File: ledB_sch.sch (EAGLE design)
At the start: 6 parts, among them IC1 LM741P

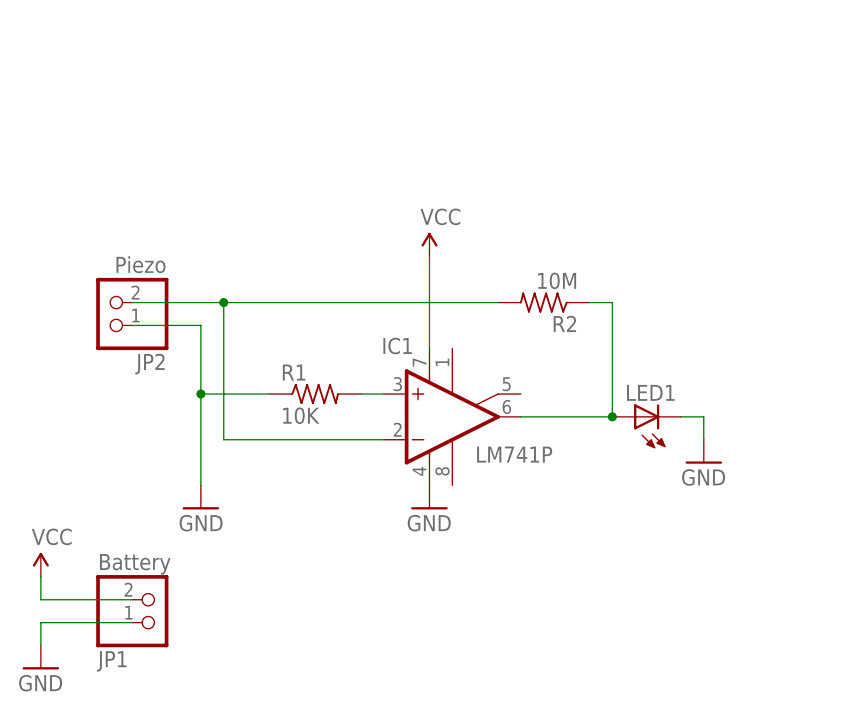
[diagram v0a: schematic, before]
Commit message: fix schema, one layer round design
and fixed the schema
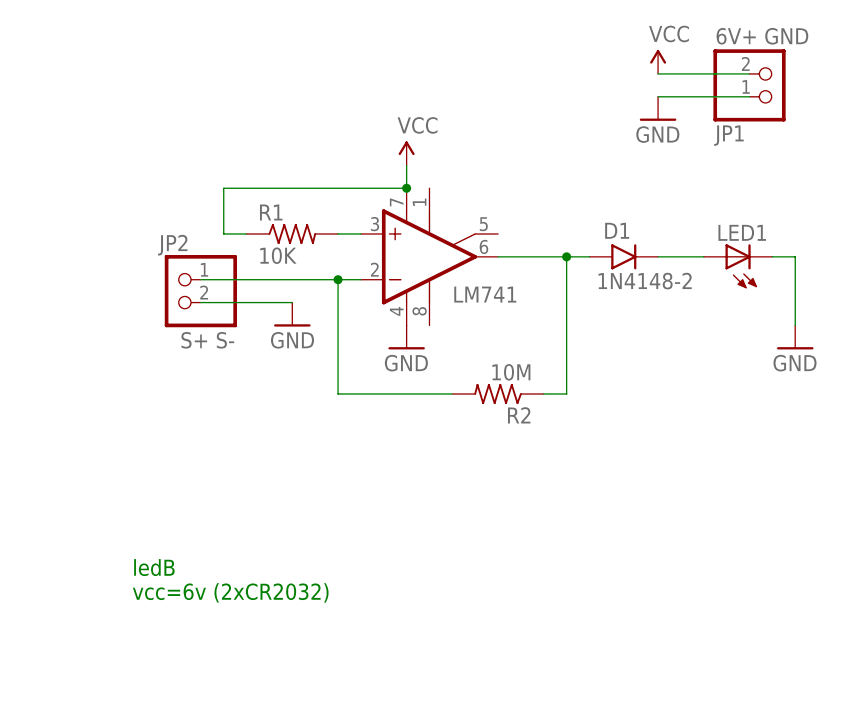
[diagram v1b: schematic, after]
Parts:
- removed IC1: LM741P, linear:LM741P
- added D1: 1N4148-2, gm-diodes:1N4148-2
- added OPAMP: LM741, linear:LM741P
- JP1: value Battery -> 6V+ GND
- JP2: value Piezo -> S+ S-
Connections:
- removed net N$3: IC1.-IN, JP2.2, R2.2
- new net N$5: D1.C, LED1.A
- new net SIG: JP2.1, OPAMP.-IN, R2.2
- net GND: now also JP2.2, OPAMP.V-; no longer IC1.V-, JP2.1, R1.1
- net N$1: now also OPAMP.+IN; no longer IC1.+IN
- net N$2: now also D1.A, OPAMP.OUT; no longer IC1.OUT, LED1.A
- net VCC: now also OPAMP.V+, R1.1; no longer IC1.V+
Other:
- note added: "ledB vcc=6v (2xCR2032)"
- moved on the sheet: JP1, JP2, LED1, R1, R2
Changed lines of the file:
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@@
 <?xml version="1.0" encoding="utf-8"?>
 <!DOCTYPE eagle SYSTEM "eagle.dtd">
-<eagle version="6.3">
+<eagle version="7.1.0">
 <drawing>
 <settings>
@@
 <setting verticaltext="up"/>
 </settings>
-<grid distance="0.1" unitdist="inch" unit="mil" style="lines" multiple="1" display="no" altdistance="0.01" altunitdist="inch" altunit="inch"/>
+<grid distance="0.1" unitdist="inch" unit="inch" style="lines" multiple="1" display="no" altdistance="0.01" altunitdist="inch" altunit="inch"/>
 <layers>
 <layer number="1" name="Top" color="4" fill="1" visible="no" active="no"/>
@@
 </classes>
 <parts>
-<part name="IC1" library="linear" deviceset="*741" device="P" technology="LM"/>
+<part name="OPAMP" library="linear" deviceset="*741" device="P" technology="LM" value="LM741"/>
 <part name="R1" library="adafruit" deviceset="R-US_" device="0207/7" value="10K"/>
 <part name="R2" library="adafruit" deviceset="R-US_" device="0207/7" value="10M"/>
 <part name="LED1" library="SparkFun-LED" deviceset="LED" device="5MM"/>
-<part name="P+1" library="SparkFun-Aesthetics" deviceset="VCC" device=""/>
-<part name="GND1" library="SparkFun-Aesthetics" deviceset="GND" device=""/>
-<part name="GND3" library="SparkFun-Aesthetics" deviceset="GND" device=""/>
 <part name="GND4" library="SparkFun-Aesthetics" deviceset="GND" device=""/>
-<part name="JP1" library="microbuilder" deviceset="HEADER-1X2" device="" value="Battery"/>
-<part name="JP2" library="microbuilder" deviceset="HEADER-1X2" device="" value="Piezo"/>
+<part name="JP1" library="microbuilder" deviceset="HEADER-1X2" device="" value="6V+     GND"/>
+<part name="JP2" library="microbuilder" deviceset="HEADER-1X2" device="" value="S+     S-"/>
 <part name="P+2" library="SparkFun-Aesthetics" deviceset="VCC" device=""/>
 <part name="GND2" library="SparkFun-Aesthetics" deviceset="GND" device=""/>
+<part name="D1" library="gm-diodes" deviceset="1N4148" device="-2"/>
+<part name="GND1" library="SparkFun-Aesthetics" deviceset="GND" device=""/>
+<part name="P+3" library="SparkFun-Aesthetics" deviceset="VCC" device=""/>
+<part name="GND3" library="SparkFun-Aesthetics" deviceset="GND" device=""/>
 </parts>
 <sheets>
 <sheet>
 <plain>
+<text x="2.54" y="0" size="1.778" layer="91">ledB
+vcc=6v (2xCR2032)</text>
 </plain>
 <instances>
-<instance part="IC1" gate="A" x="38.1" y="20.32" smashed="yes">
-<attribute name="NAME" x="30.226" y="27.305" size="1.778" layer="95"/>
-<attribute name="VALUE" x="40.64" y="15.24" size="1.778" layer="96"/>
+<instance part="OPAMP" gate="A" x="35.56" y="38.1" smashed="yes">
+<attribute name="VALUE" x="38.1" y="33.02" size="1.778" layer="96"/>
 </instance>
-<instance part="R1" gate="G$1" x="22.86" y="22.86"/>
-<instance part="R2" gate="G$1" x="48.26" y="33.02" rot="R180"/>
-<instance part="LED1" gate="G$1" x="58.42" y="20.32" rot="R90"/>
-<instance part="P+1" gate="1" x="35.56" y="38.1"/>
-<instance part="GND1" gate="1" x="10.16" y="10.16" rot="MR0"/>
-<instance part="GND3" gate="1" x="35.56" y="10.16"/>
-<instance part="GND4" gate="1" x="66.04" y="15.24"/>
-<instance part="JP1" gate="G$1" x="5.08" y="0" rot="MR180"/>
-<instance part="JP2" gate="G$1" x="0" y="33.02" rot="R180"/>
-<instance part="P+2" gate="1" x="-7.62" y="2.54"/>
-<instance part="GND2" gate="1" x="-7.62" y="-7.62"/>
+<instance part="R1" gate="G$1" x="20.32" y="40.64"/>
+<instance part="R2" gate="G$1" x="43.18" y="22.86" rot="R180"/>
+<instance part="LED1" gate="G$1" x="68.58" y="38.1" rot="R90"/>
+<instance part="GND4" gate="1" x="76.2" y="27.94"/>
+<instance part="JP1" gate="G$1" x="73.66" y="58.42" rot="MR180"/>
+<instance part="JP2" gate="G$1" x="7.62" y="33.02" smashed="yes" rot="MR0">
+<attribute name="NAME" x="8.89" y="38.735" size="1.778" layer="95" rot="MR0"/>
+<attribute name="VALUE" x="13.97" y="27.94" size="1.778" layer="96" rot="MR0"/>
+</instance>
+<instance part="P+2" gate="1" x="60.96" y="58.42"/>
+<instance part="GND2" gate="1" x="60.96" y="53.34"/>
+<instance part="D1" gate="G$1" x="58.42" y="38.1"/>
+<instance part="GND1" gate="1" x="20.32" y="30.48" rot="MR0"/>
+<instance part="P+3" gate="1" x="33.02" y="48.26"/>
+<instance part="GND3" gate="1" x="33.02" y="27.94"/>
 </instances>
 <busses>
 </busses>
 <nets>
-<net name="N$1" class="0">
-<segment>
-<pinref part="IC1" gate="A" pin="+IN"/>
-<pinref part="R1" gate="G$1" pin="2"/>
-<wire x1="27.94" y1="22.86" x2="30.48" y2="22.86" width="0.1524" layer="91"/>
-</segment>
-</net>
 <net name="GND" class="0">
 <segment>
-<pinref part="R1" gate="G$1" pin="1"/>
-<pinref part="JP2" gate="G$1" pin="1"/>
-<pinref part="GND1" gate="1" pin="GND"/>
-<wire x1="2.54" y1="30.48" x2="10.16" y2="30.48" width="0.1524" layer="91"/>
-<wire x1="10.16" y1="30.48" x2="10.16" y2="22.86" width="0.1524" layer="91"/>
-<wire x1="10.16" y1="22.86" x2="10.16" y2="12.7" width="0.1524" layer="91"/>
-<wire x1="17.78" y1="22.86" x2="10.16" y2="22.86" width="0.1524" layer="91"/>
-<junction x="10.16" y="22.86"/>
-</segment>
-<segment>
-<pinref part="IC1" gate="A" pin="V-"/>
+<pinref part="OPAMP" gate="A" pin="V-"/>
 <pinref part="GND3" gate="1" pin="GND"/>
 </segment>
@@
 <pinref part="LED1" gate="G$1" pin="C"/>
 <pinref part="GND4" gate="1" pin="GND"/>
-<wire x1="66.04" y1="17.78" x2="66.04" y2="20.32" width="0.1524" layer="91"/>
-<wire x1="66.04" y1="20.32" x2="63.5" y2="20.32" width="0.1524" layer="91"/>
+<wire x1="76.2" y1="30.48" x2="76.2" y2="38.1" width="0.1524" layer="91"/>
+<wire x1="76.2" y1="38.1" x2="73.66" y2="38.1" width="0.1524" layer="91"/>
 </segment>
 <segment>
 <pinref part="JP1" gate="G$1" pin="1"/>
 <pinref part="GND2" gate="1" pin="GND"/>
-<wire x1="2.54" y1="-2.54" x2="-7.62" y2="-2.54" width="0.1524" layer="91"/>
-<wire x1="-7.62" y1="-2.54" x2="-7.62" y2="-5.08" width="0.1524" layer="91"/>
+<wire x1="71.12" y1="55.88" x2="60.96" y2="55.88" width="0.1524" layer="91"/>
+</segment>
+<segment>
+<pinref part="GND1" gate="1" pin="GND"/>
+<pinref part="JP2" gate="G$1" pin="2"/>
+<wire x1="20.32" y1="33.02" x2="10.16" y2="33.02" width="0.1524" layer="91"/>
 </segment>
 </net>
 <net name="VCC" class="0">
-<segment>
-<pinref part="IC1" gate="A" pin="V+"/>
-<pinref part="P+1" gate="1" pin="VCC"/>
-<wire x1="35.56" y1="38.1" x2="35.56" y2="27.94" width="0.1524" layer="91"/>
-</segment>
 <segment>
 <pinref part="JP1" gate="G$1" pin="2"/>
 <pinref part="P+2" gate="1" pin="VCC"/>
-<wire x1="2.54" y1="0" x2="-7.62" y2="0" width="0.1524" layer="91"/>
-<wire x1="-7.62" y1="0" x2="-7.62" y2="2.54" width="0.1524" layer="91"/>
+<wire x1="71.12" y1="58.42" x2="60.96" y2="58.42" width="0.1524" layer="91"/>
+</segment>
+<segment>
+<pinref part="R1" gate="G$1" pin="1"/>
+<wire x1="12.7" y1="45.72" x2="12.7" y2="40.64" width="0.1524" layer="91"/>
+<wire x1="12.7" y1="40.64" x2="15.24" y2="40.64" width="0.1524" layer="91"/>
+<pinref part="OPAMP" gate="A" pin="V+"/>
+<wire x1="12.7" y1="45.72" x2="33.02" y2="45.72" width="0.1524" layer="91"/>
+<pinref part="P+3" gate="1" pin="VCC"/>
+<wire x1="33.02" y1="48.26" x2="33.02" y2="45.72" width="0.1524" layer="91"/>
+<junction x="33.02" y="45.72"/>
 </segment>
 </net>
 <net name="N$2" class="0">
 <segment>
-<pinref part="IC1" gate="A" pin="OUT"/>
 <pinref part="R2" gate="G$1" pin="1"/>
-<wire x1="53.34" y1="33.02" x2="55.88" y2="33.02" width="0.1524" layer="91"/>
-<wire x1="55.88" y1="33.02" x2="55.88" y2="20.32" width="0.1524" layer="91"/>
-<wire x1="55.88" y1="20.32" x2="45.72" y2="20.32" width="0.1524" layer="91"/>
+<pinref part="D1" gate="G$1" pin="A"/>
+<pinref part="OPAMP" gate="A" pin="OUT"/>
+<wire x1="53.34" y1="38.1" x2="50.8" y2="38.1" width="0.1524" layer="91"/>
+<wire x1="50.8" y1="38.1" x2="43.18" y2="38.1" width="0.1524" layer="91"/>
+<wire x1="48.26" y1="22.86" x2="50.8" y2="22.86" width="0.1524" layer="91"/>
+<wire x1="50.8" y1="22.86" x2="50.8" y2="38.1" width="0.1524" layer="91"/>
+<junction x="50.8" y="38.1"/>
+</segment>
+</net>
+<net name="N$5" class="0">
+<segment>
 <pinref part="LED1" gate="G$1" pin="A"/>
-<junction x="55.88" y="20.32"/>
-</segment>
-</net>
-<net name="N$3" class="0">
-<segment>
-<pinref part="IC1" gate="A" pin="-IN"/>
-<wire x1="12.7" y1="33.02" x2="12.7" y2="17.78" width="0.2032" layer="91"/>
-<wire x1="12.7" y1="17.78" x2="30.48" y2="17.78" width="0.2032" layer="91"/>
+<pinref part="D1" gate="G$1" pin="C"/>
+<wire x1="60.96" y1="38.1" x2="66.04" y2="38.1" width="0.1524" layer="91"/>
+</segment>
+</net>
+<net name="SIG" class="0">
+<segment>
+<pinref part="OPAMP" gate="A" pin="-IN"/>
+<wire x1="38.1" y1="22.86" x2="25.4" y2="22.86" width="0.2032" layer="91"/>
+<wire x1="25.4" y1="22.86" x2="25.4" y2="35.56" width="0.2032" layer="91"/>
+<wire x1="25.4" y1="35.56" x2="27.94" y2="35.56" width="0.2032" layer="91"/>
 <pinref part="R2" gate="G$1" pin="2"/>
-<wire x1="12.7" y1="33.02" x2="43.18" y2="33.02" width="0.2032" layer="91"/>
-<pinref part="JP2" gate="G$1" pin="2"/>
-<wire x1="12.7" y1="33.02" x2="2.54" y2="33.02" width="0.1524" layer="91"/>
-<junction x="12.7" y="33.02"/>
+<wire x1="10.16" y1="35.56" x2="25.4" y2="35.56" width="0.1524" layer="91"/>
+<junction x="25.4" y="35.56"/>
+<pinref part="JP2" gate="G$1" pin="1"/>
+</segment>
+</net>
+<net name="N$1" class="0">
+<segment>
+<pinref part="OPAMP" gate="A" pin="+IN"/>
+<pinref part="R1" gate="G$1" pin="2"/>
+<wire x1="25.4" y1="40.64" x2="27.94" y2="40.64" width="0.1524" layer="91"/>
 </segment>
 </net>
@@
 </schematic>
 </drawing>
+<compatibility>
+<note version="6.3" minversion="6.2.2" severity="warning">
+Since Version 6.2.2 text objects can contain more than one line,
+which will not be processed correctly with this version.
+</note>
+</compatibility>
 </eagle>
